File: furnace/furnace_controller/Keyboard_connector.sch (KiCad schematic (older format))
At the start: 1 part

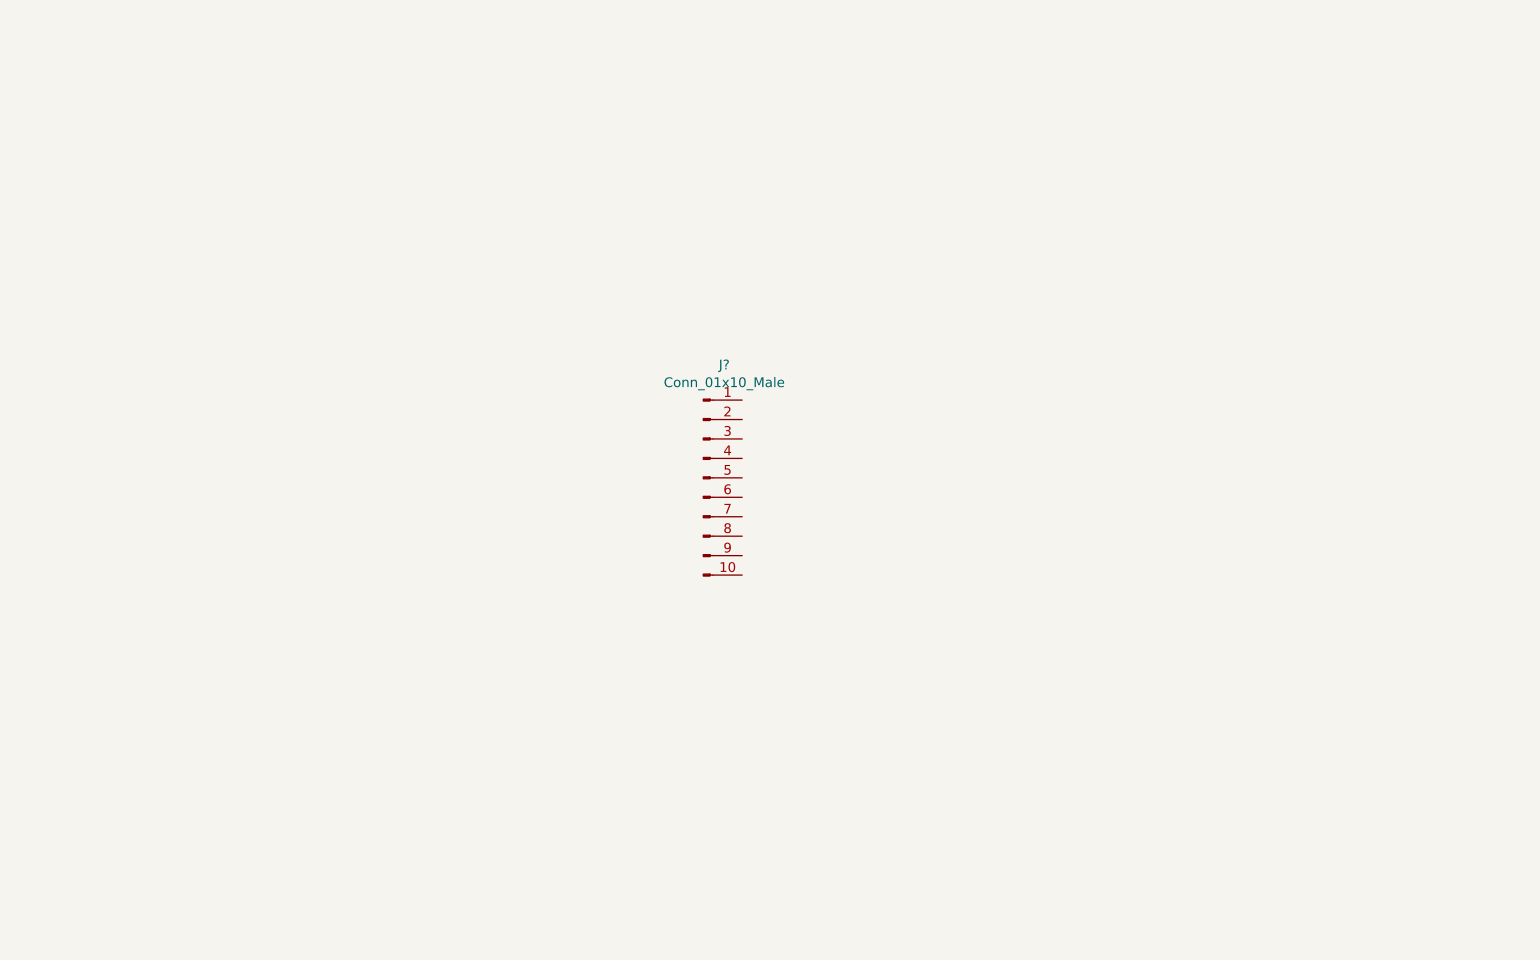
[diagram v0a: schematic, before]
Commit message: Add files via upload
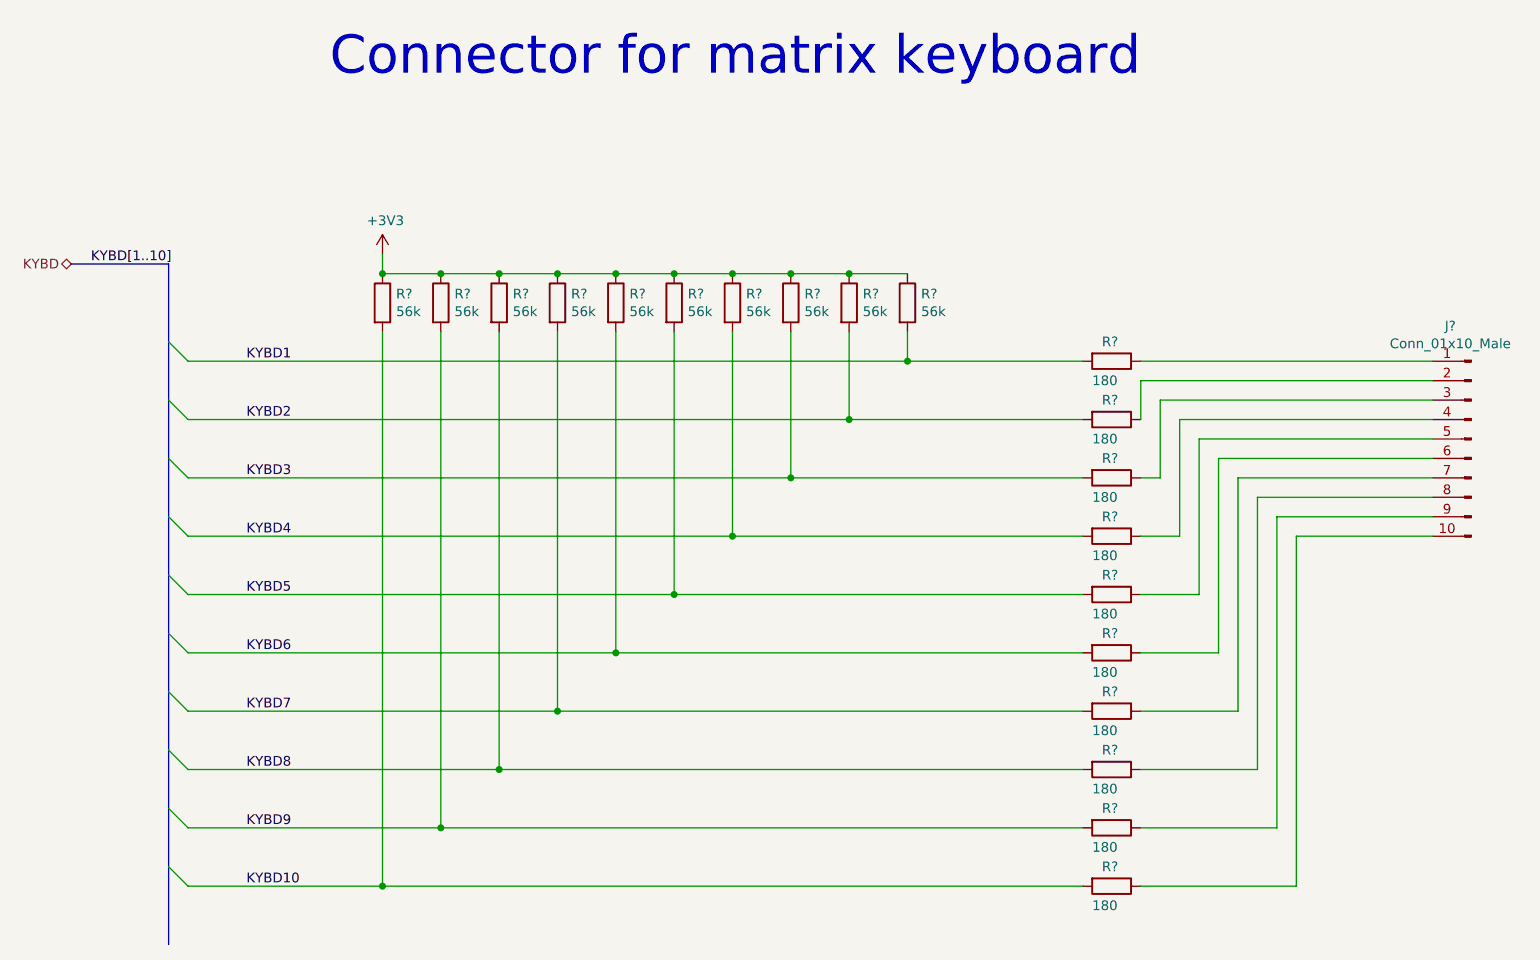
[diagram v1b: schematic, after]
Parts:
- added R? (x10): 180, Resistor_SMD:R_0603_1608Metric_Pad0.98x0.95mm_HandSolder, symbol Device:R
- added R? (x10): 56k, Resistor_SMD:R_0603_1608Metric_Pad0.98x0.95mm_HandSolder, symbol Device:R
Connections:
- net at J?.1 (Pin_1): now also R?.1
- net at J?.10 (Pin_10): now also R?.1
- net at J?.2 (Pin_2): now also R?.1
- net at J?.3 (Pin_3): now also R?.1
- net at J?.4 (Pin_4): now also R?.1
- net at J?.5 (Pin_5): now also R?.1
- net at J?.6 (Pin_6): now also R?.1
- net at J?.7 (Pin_7): now also R?.1
- net at J?.8 (Pin_8): now also R?.1
- net at J?.9 (Pin_9): now also R?.1
- new net +3V3: R?.1, R?.1, R?.1, R?.1, R?.1, R?.1, R?.1, R?.1, R?.1, R?.1
- new net KYBD1: R?.2, R?.2
- new net KYBD10: R?.2, R?.2
- new net KYBD2: R?.2, R?.2
- new net KYBD3: R?.2, R?.2
- new net KYBD4: R?.2, R?.2
- new net KYBD5: R?.2, R?.2
- new net KYBD6: R?.2, R?.2
- new net KYBD7: R?.2, R?.2
- new net KYBD8: R?.2, R?.2
- new net KYBD9: R?.2, R?.2
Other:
- note added: "Connector for matrix keyboard"
- moved on the sheet: J?
